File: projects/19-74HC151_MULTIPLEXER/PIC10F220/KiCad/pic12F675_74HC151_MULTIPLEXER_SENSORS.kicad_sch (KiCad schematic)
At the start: 13 parts, among them M1 Motor_DC, M2 Motor_DC, Q1 NMOS, Q2 NMOS, U1 PIC12F675-IP, U2 74151, U3 LM35-LP, U4 A1369xUA-10, U5 LM35-LP, U6 A1369xUA-10

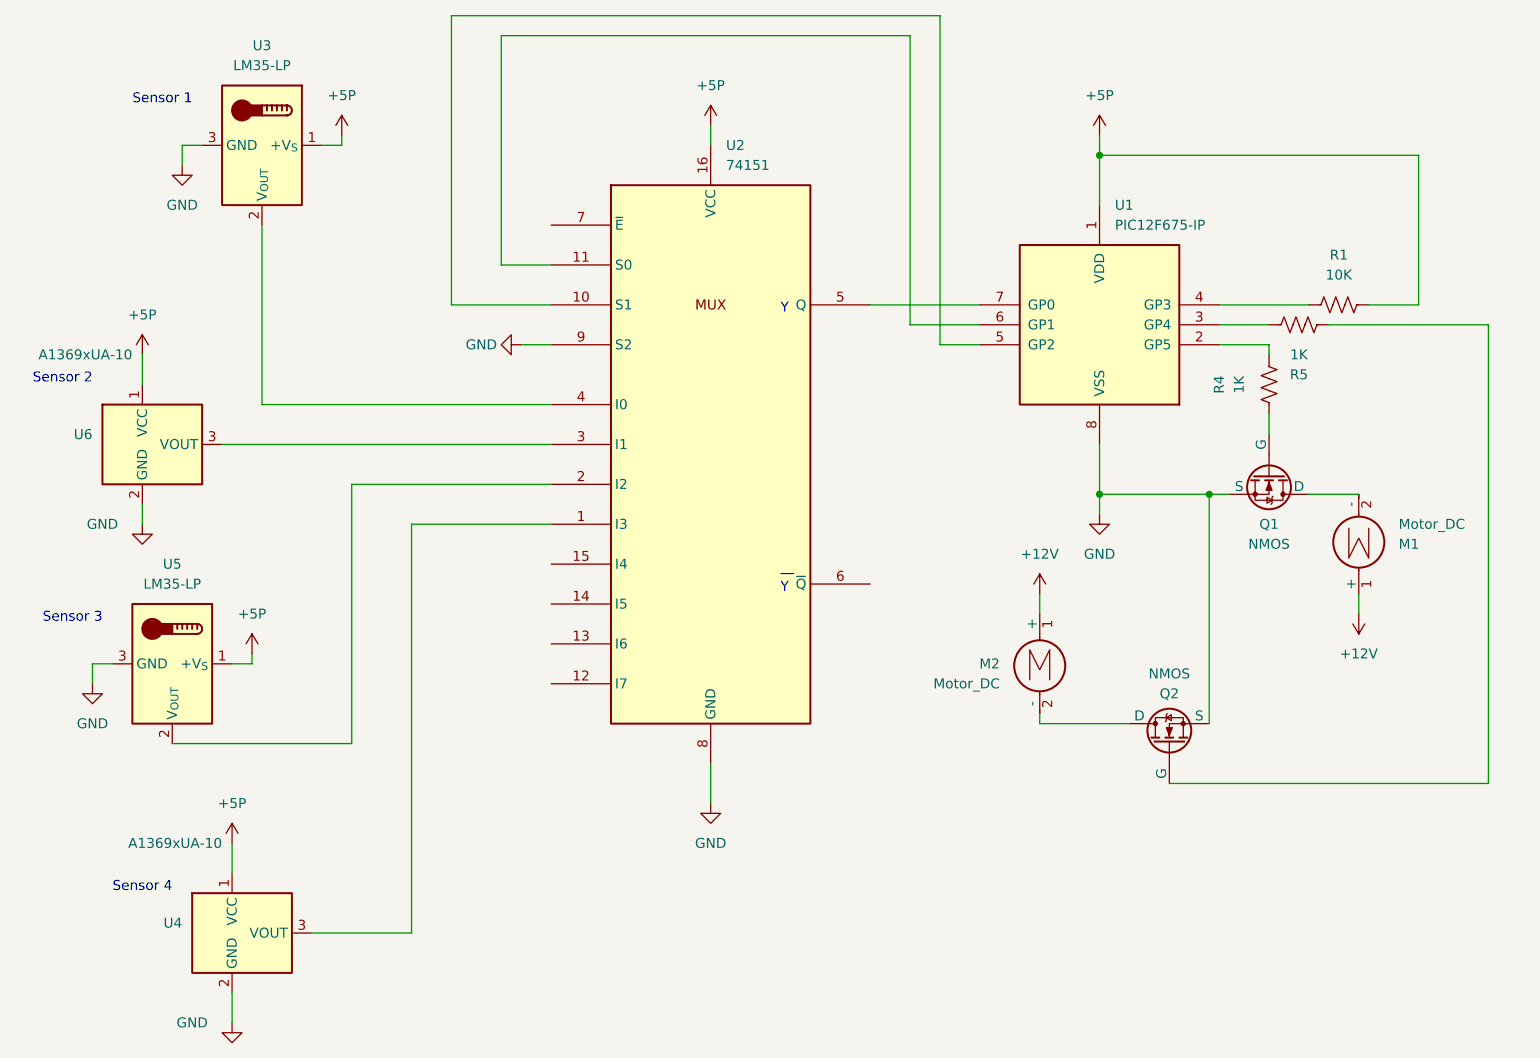
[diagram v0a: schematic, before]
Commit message: Doc
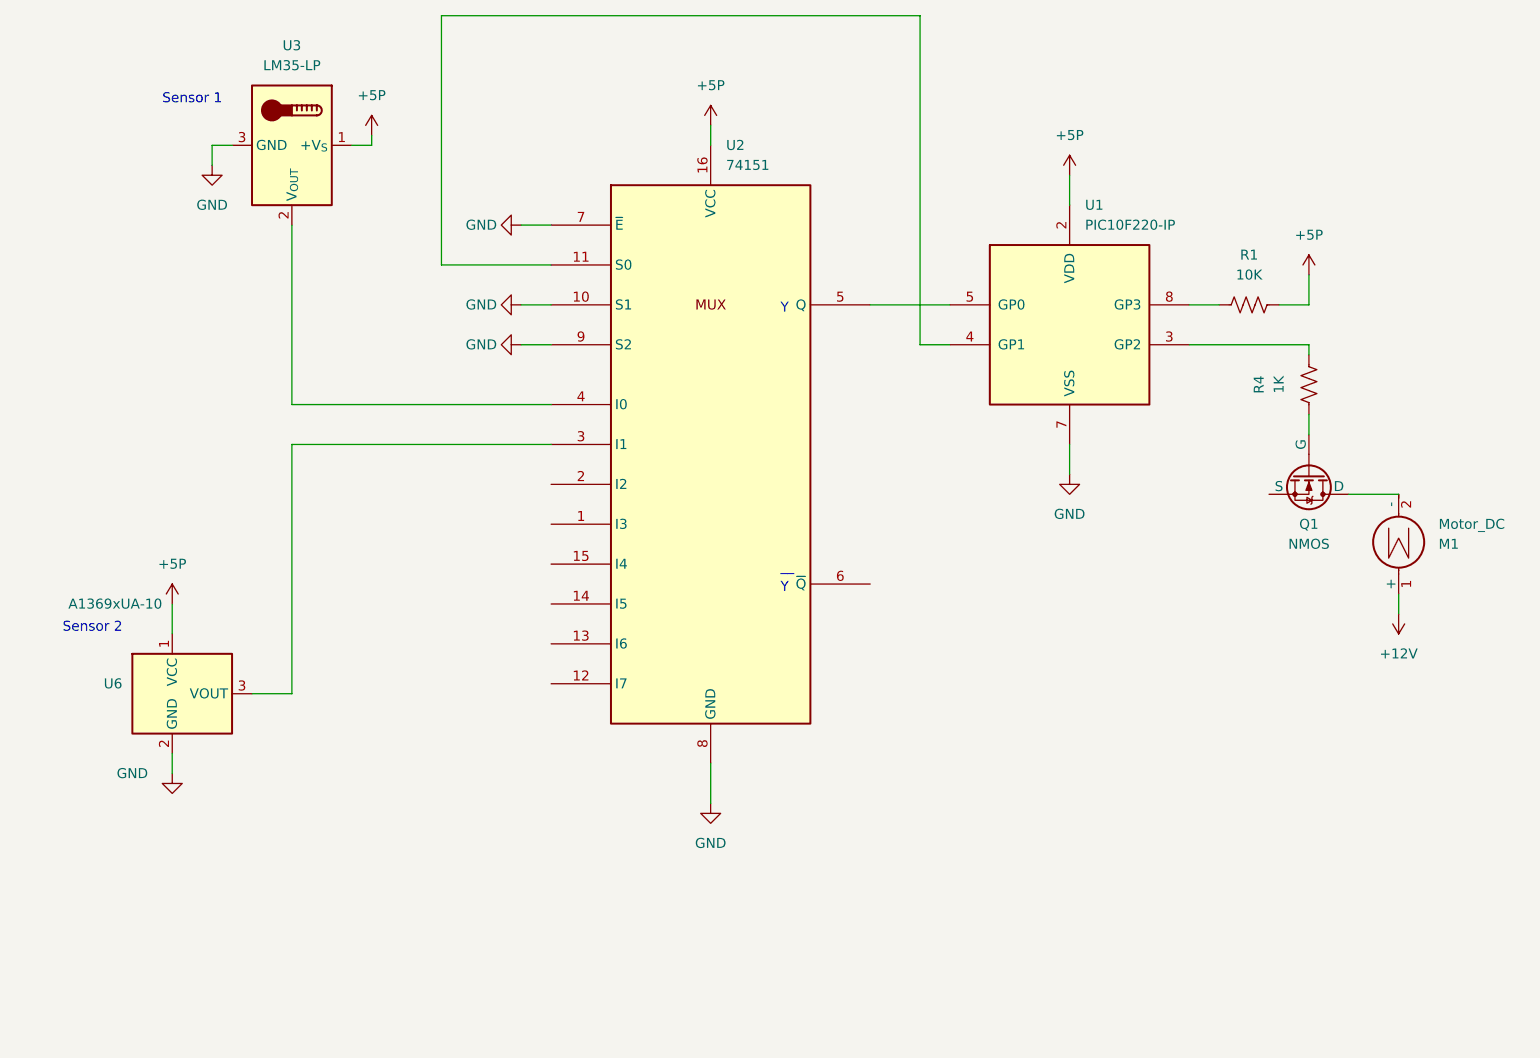
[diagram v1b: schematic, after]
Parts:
- removed M2: Motor_DC, symbol Motor:Motor_DC
- removed Q2: NMOS, symbol Simulation_SPICE:NMOS
- removed R5: 1K, symbol Device:R_US
- removed U1: PIC12F675-IP, Package_DIP:DIP-8_W7.62mm, symbol MCU_Microchip_PIC12:PIC12F675-IP
- removed U4: A1369xUA-10, Sensor_Current:Allegro_SIP-3, symbol Sensor_Current:A1369xUA-10
- removed U5: LM35-LP, Package_TO_SOT_THT:TO-92_Inline, symbol Sensor_Temperature:LM35-LP
- added U1: PIC10F220-IP, Package_DIP:DIP-8_W7.62mm, symbol MCU_Microchip_PIC10:PIC10F220-IP
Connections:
- net +5P: now also U1.2 (VDD)
- net GND: now also U2.10 (S1), U2.7 (~{E}), U1.7 (VSS); no longer Q1.3 (S)
- net at R1.1: now also U1.8 (GP3)
- net at U2.11 (S0): now also U1.4 (GP1)
- net at U2.5 (Q): now also U1.5 (GP0)
- net at R4.2: now also U1.3 (GP2)
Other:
- note removed: "Sensor 3"
- note removed: "Sensor 4"
- title: PIC10F220 and 74HC151 monitoring 4 sensors -> PIC10F220 and 74HC151 monitoring 2 sensors
- moved on the sheet: M1, Q1, R1, R4, U3, U6
